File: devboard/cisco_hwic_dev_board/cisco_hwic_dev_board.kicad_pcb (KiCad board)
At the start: 2 copper layers, 3 parts, among them J1 Conn_02x20_Odd_Even, J2 Conn_02x34_Top_Bottom_Cisco, J3 Conn_01x15

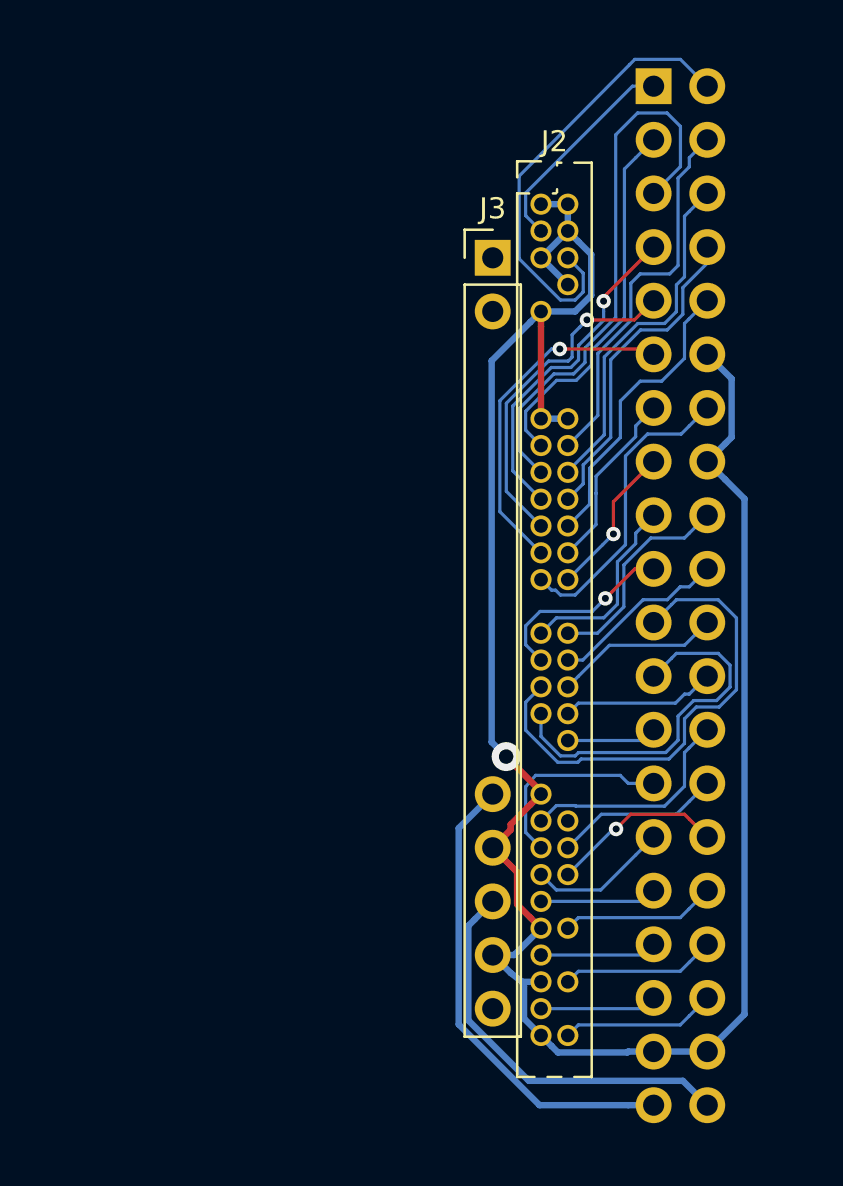
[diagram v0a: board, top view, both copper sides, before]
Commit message: First version.
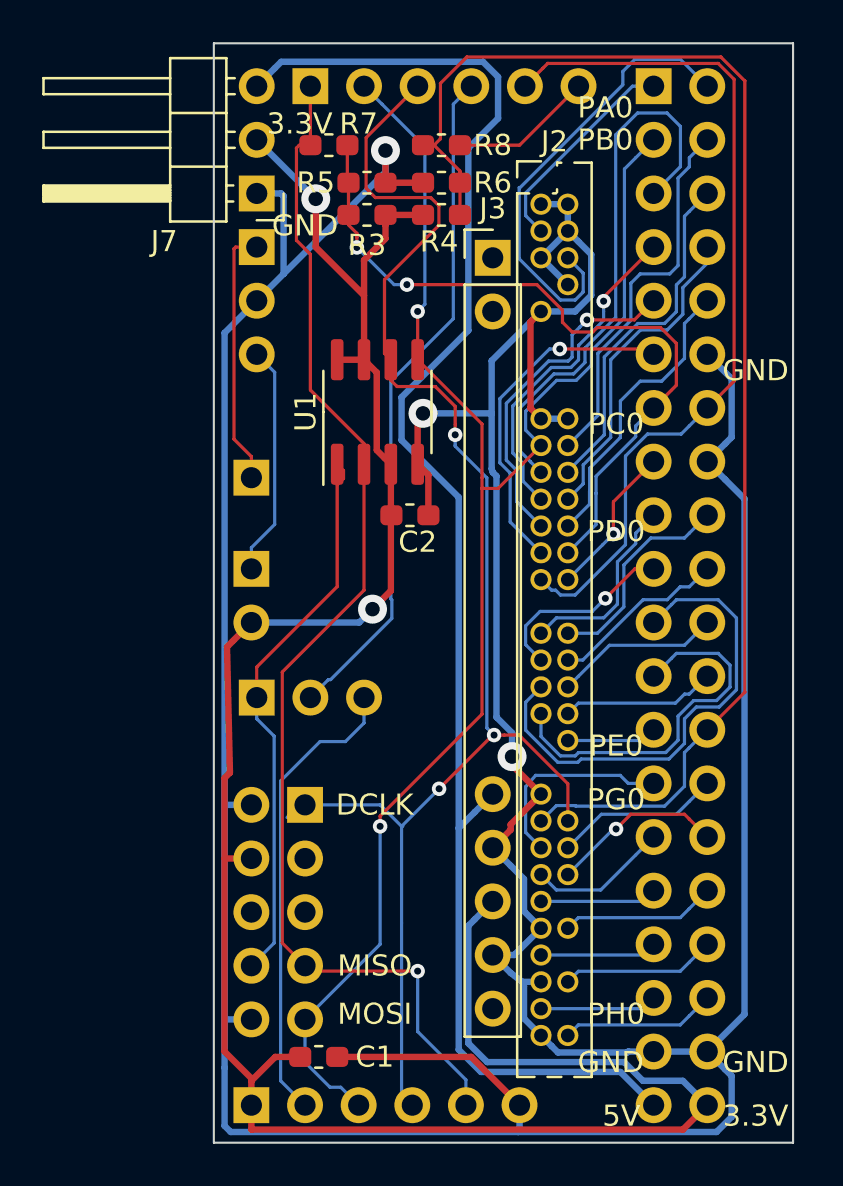
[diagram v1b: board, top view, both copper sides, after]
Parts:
- added C1: C, Capacitor_SMD:C_0603_1608Metric_Pad1.05x0.95mm_HandSolder, F.Cu at (-551.3, -538.7)
- added C2: C, Capacitor_SMD:C_0603_1608Metric_Pad1.05x0.95mm_HandSolder, F.Cu at (-547.0, -564.4)
- added J4: USB Blaster Active Serial, Connector_PinHeader_2.54mm:PinHeader_2x05_P2.54mm_Vertical, B.Cu at (-551.9, -550.7)
- added J5: ATT85_VIN, Connector_PinHeader_2.54mm:PinHeader_1x01_P2.54mm_Vertical, B.Cu at (-554.5, -566.2)
- added J6: SD Card, Connector_PinHeader_2.54mm:PinHeader_1x06_P2.54mm_Vertical, B.Cu at (-554.5, -536.4)
- added J7: Power, Connector_PinHeader_2.54mm:PinHeader_1x03_P2.54mm_Horizontal, F.Cu at (-554.2, -579.6)
- added JP1: 3.3V Main, Connector_PinHeader_2.54mm:PinHeader_2x01_P2.54mm_Vertical, B.Cu at (-554.5, -561.8)
- added JP2: Jumper_3_Bridged12, Connector_PinHeader_2.54mm:PinHeader_1x03_P2.54mm_Vertical, B.Cu at (-554.2, -555.8)
- added R3: NS, Resistor_SMD:R_0603_1608Metric_Pad1.05x0.95mm_HandSolder, F.Cu at (-549.0, -578.6)
- added R4: NS, Resistor_SMD:R_0603_1608Metric_Pad1.05x0.95mm_HandSolder, F.Cu at (-545.5, -578.6)
- added R5: NS, Resistor_SMD:R_0603_1608Metric_Pad1.05x0.95mm_HandSolder, F.Cu at (-549.0, -580.1)
- added R6: NS, Resistor_SMD:R_0603_1608Metric_Pad1.05x0.95mm_HandSolder, F.Cu at (-545.5, -580.1)
- added R7: NS, Resistor_SMD:R_0603_1608Metric_Pad1.05x0.95mm_HandSolder, F.Cu at (-550.8, -581.9)
- added R8: NS, Resistor_SMD:R_0603_1608Metric_Pad1.05x0.95mm_HandSolder, F.Cu at (-545.5, -581.9)
- added U1: AT25xxx, Package_SO:SOIC-8_3.9x4.9mm_P1.27mm, F.Cu at (-548.5, -569.3)
- added U2: ATtiny85_devboard, cisco_hwic_dev_board:Digispark_ATtiny85, B.Cu at (-551.7, -584.7)
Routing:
- net GND: track 103.9 -> 211.8 mm, vias 1 -> 3
- net +3V3: track 19.1 -> 109.5 mm, vias 0 -> 2
- net /DCLK: track 0.00 -> 71.0 mm, vias 0 -> 3
- net /DATA0: track 17.8 -> 77.2 mm, vias 0 -> 2
- net /SPI_MISO: track 0.00 -> 58.3 mm, vias 0 -> 1
- net /DCLK_OE_: track 10.6 -> 64.9 mm
- net +5V: track 22.4 -> 73.9 mm
- net /SPISD_CSN: track 0.00 -> 32.2 mm
- net /PC1: track 14.3 -> 41.1 mm
- net /SPI_CSN: track 0.00 -> 26.4 mm
- net /PC0: track 8.54 -> 34.6 mm, vias 0 -> 2
- net /SD_CSN: track 0.00 -> 22.1 mm
- net Net-(J5-Pad1): track 0.00 -> 12.3 mm
- net Net-(JP1-Pad1): track 0.00 -> 11.0 mm
- net Net-(R8-Pad2): track 0.00 -> 6.77 mm
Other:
- board outline added: 27.4 x 52.1 mm
- board text added: "3.3V"
- board text added: "5V"
- board text added: "DCLK"
- board text added: "GND"
- board text added: "MISO"
- board text added: "MOSI"
- board text added: "PA0"
- board text added: "PB0"
- board text added: "PC0"
- board text added: "PD0"
- board text added: "PE0"
- board text added: "PG0"
- board text added: "PH0"
